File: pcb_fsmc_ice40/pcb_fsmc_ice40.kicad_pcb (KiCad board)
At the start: 2 copper layers, 76.2 x 32 mm, 44 parts, among them P2 CONN_01X20, P3 CONN_01X20, P4 MICRO-SD, P5 CONN_01X12, P6 CONN_01X12, P7 KNUSB, U1 STM32F40X_LQFP144, X1 CRYSTAL

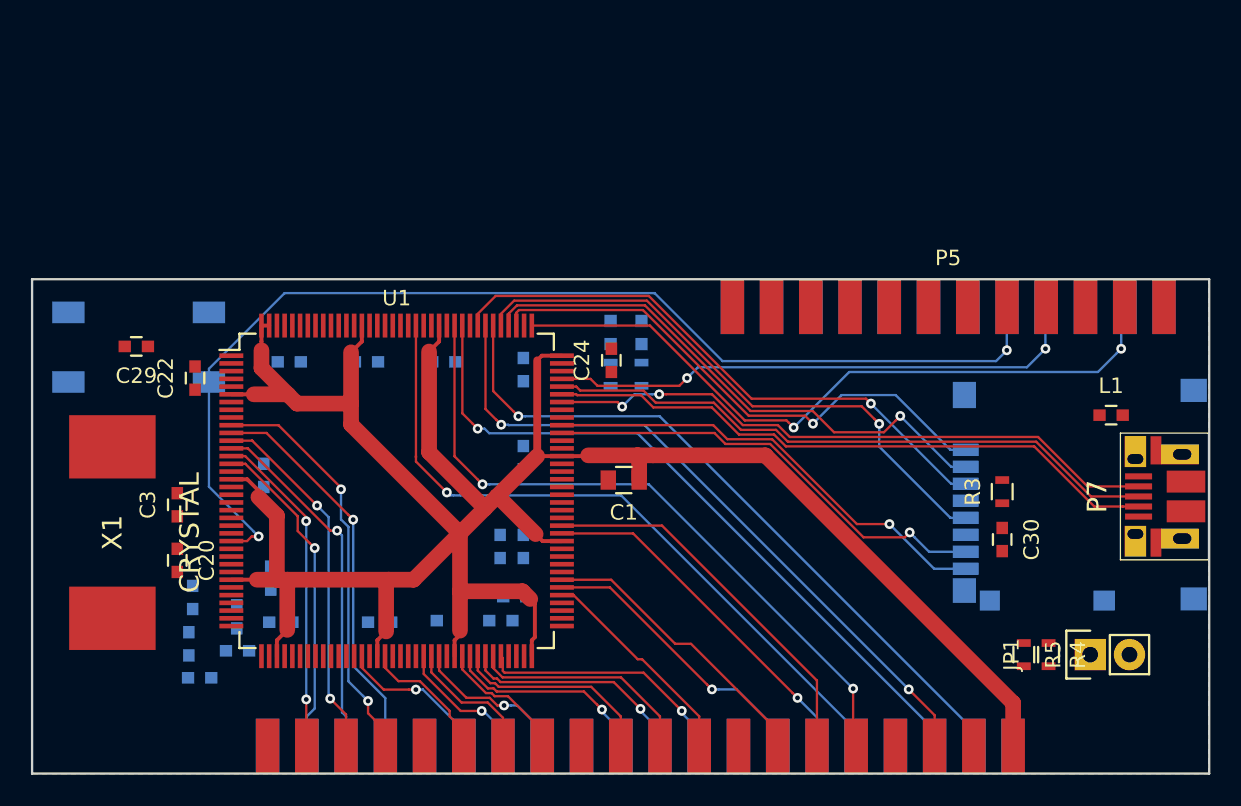
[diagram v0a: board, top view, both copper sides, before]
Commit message: Mostly complete routing.
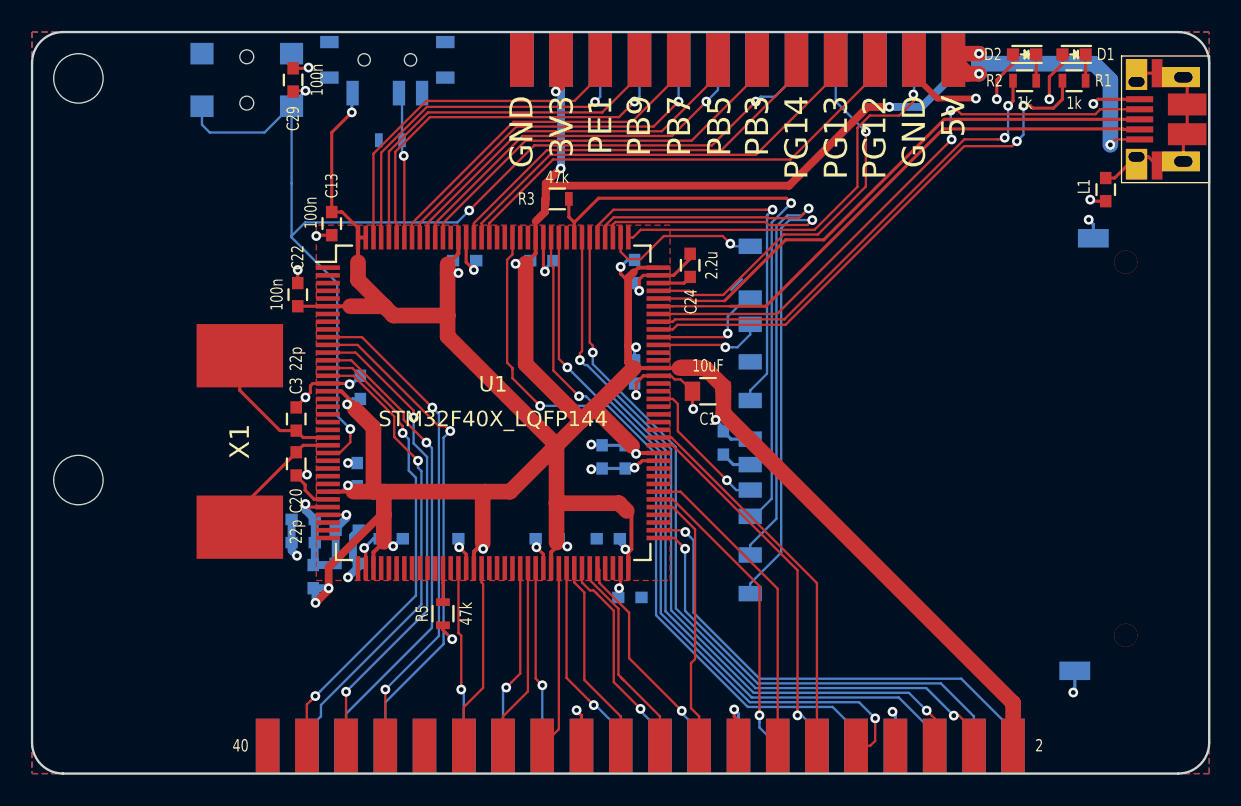
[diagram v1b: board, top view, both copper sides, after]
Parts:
- removed JP1: Jumper_NO_Small, Pin_Headers:Pin_Header_Straight_1x02
- removed P3: CONN_01X20, knielsenlib:ice40_vert_conn
- removed P4: MICRO-SD, knielsenlib:SD_502774
- removed P6: CONN_01X12, knielsenlib:ice40_top_conn_12
- added P1: SD_CARD, knielsenlib:SD_CARD_10100, B.Cu at (170.8, 111.7)
- added REF**: MountingHole_3.2mm_M3, Mounting_Holes:MountingHole_3.2mm_M3, F.Cu at (103.0, 87.0)
- added REF**: MountingHole_3.2mm_M3, Mounting_Holes:MountingHole_3.2mm_M3, F.Cu at (103.0, 113.0)
- added SW1: SWITCH_INV, knielsenlib:switch_msk_12c02, B.Cu at (123.0, 85.8)
- B1: footprint knielsenlib:SWITCH_FSMJSMA -> knielsenlib:pushbutton_EVQ_PSR02K
- C13, D1, D2, R1, R2: moved to F.Cu
- C30, R4: moved to B.Cu
- P2: value CONN_01X20 -> CONN_02X20; moved to F.Cu
- P5: value CONN_01X12 -> CONN_02X12
- moved R4 54.1 mm to (123.2, 91.0), turned to 180 degrees
- moved R5 37.7 mm to (126.6, 121.7), turned to 90 degrees
- moved R3 34.5 mm to (134.0, 94.8), turned to 0 degrees
- moved R1 33.8 mm to (167.4, 87.2), turned to 0 degrees
- moved D1 33.3 mm to (167.4, 85.5), turned to 180 degrees
- moved R2 32.9 mm to (164.2, 87.2), turned to 0 degrees
- moved D2 32.3 mm to (164.2, 85.5), turned to 180 degrees
- moved P7 24.4 mm to (174.5, 89.7)
- moved P5 21.0 mm to (145.7, 85.8), turned to 0 degrees
- moved C29 20.0 mm to (116.9, 87.1), turned to 90 degrees
- moved C30 19.1 mm to (144.8, 110.6)
- moved B1 18.7 mm to (113.9, 87.1), turned to 90 degrees
- moved L1 14.6 mm to (169.5, 94.2), turned to 90 degrees
- moved X1 10.1 mm to (113.5, 110.5)
- moved C20 9.92 mm to (117.1, 112.0)
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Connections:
- P2 pad 10: /sram_d10 -> /sram_we
- P2 pad 11: /sram_d8 -> /sram_d0
- P2 pad 12: GND -> /sram_d1
- P2 pad 13: /sram_d6 -> /sram_d14
- P2 pad 14: /sram_d4 -> /sram_d15
- P2 pad 15: /sram_a6 -> GND
- P2 pad 17: /sram_a1 -> /sram_d12
- P2 pad 18: /sram_a3 -> /sram_d13
- P2 pad 19: /sram_a5 -> /sram_d10
- P2 pad 2: /sram_d2 -> +3.3V
- P2 pad 20: GND -> /sram_d11
- P2 pad 3: /sram_oe -> /fpga_io1
- P2 pad 4: GND -> /sram_d2
- P2 pad 5: /sram2_ce -> /sram_oe
- P2 pad 6: /sram_d0 -> /sram_d3
- P2 pad 7: /sram_d14 -> GND
- P2 pad 9: /sram_d12 -> /sram2_ce
- P5 pad 1: Net-(P5-Pad1) -> GND
- P5 pad 10: Net-(P5-Pad10) -> /pb7
- P5 pad 11: Net-(P5-Pad11) -> /pb4
- P5 pad 12: Net-(P5-Pad12) -> /pb5
- P5 pad 2: Net-(P5-Pad2) -> GND
- P5 pad 3: Net-(P5-Pad3) -> +3.3V
- P5 pad 4: Net-(P5-Pad4) -> +3.3V
- P5 pad 5: Net-(P5-Pad5) -> /pe0
- P5 pad 6: Net-(P5-Pad6) -> /pe1
- P5 pad 7: Net-(P5-Pad7) -> /pb8
- P5 pad 8: Net-(P5-Pad8) -> /pb9
- P5 pad 9: Net-(P5-Pad9) -> /pb6
- R1 pad 1: +3.3V -> /user_led1
- R2 pad 1: /user_led -> /user_led2
- R4 pad 1: GND -> /boot0
- R4 pad 2: /boot0 -> GND
- U1 pad 100: /pa8 -> /user_led1
- U1 pad 101: /pa9 -> /user_led2
- U1 pad 110: /pa15 -> /sd_wp
- U1 pad 127: /sram4_ce -> /pg12
- U1 pad 132: /user_led -> /pg15
- U1 pad 133: /swo -> /pb3
- U1 pad 141: /sram_ble -> /pe0
- U1 pad 142: /sram_bhe -> /pe1
- U1 pad 7: /sd_cd -> /pc13
- U1 pad 73: /pb12 -> /fpga_io1
- U1 pad 74: /pb13 -> /fpga_io2
- U1 pad 8: /sd_wp -> /pc14
- U1 pad 91: /pg6 -> /sd_cd
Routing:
- net +3.3V: track 157.9 -> 250.6 mm, vias 0 -> 19
- net GND: track 0.00 -> 80.6 mm, vias 0 -> 30
- net /user_led1: track 0.00 -> 34.7 mm, vias 0 -> 2
- net /fpga_io2: track 0.00 -> 32.1 mm, vias 0 -> 1
- net /user_led2: track 0.00 -> 31.3 mm, vias 0 -> 2
- net /pg12: track 0.00 -> 30.8 mm
- net /fpga_io1: track 0.00 -> 29.5 mm, vias 0 -> 1
- net /pg13: track 0.00 -> 28.8 mm
- net /pg14: track 0.00 -> 26.8 mm
- net /pb3: track 0.00 -> 26.2 mm
- net /pb8: track 0.00 -> 25.2 mm, vias 0 -> 1
- net /pb9: track 0.00 -> 24.8 mm
- net /pb4: track 0.00 -> 24.7 mm, vias 0 -> 1
- net /pb5: track 0.00 -> 24.7 mm
- net /pb6: track 0.00 -> 23.6 mm, vias 0 -> 1
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- added copper zone on F.Cu, net +3.3V
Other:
- board size 76.2 x 32 mm -> 76.2 x 48 mm
- board text added: "1"
- board text added: "2"
- board text added: "39"
- board text added: "3V3"
- board text added: "40"
- board text added: "5V"
- board text added: "GND"
- board text added: "NRST"
- board text added: "PB3"
- board text added: "PB4"
- board text added: "PB5"
- board text added: "PB6"
- board text added: "PB7"
- board text added: "PB8"
- board text added: "PB9"
- board text added: "PE0"
- board text added: "PE1"
- board text added: "PG12"
- board text added: "PG13"
- board text added: "PG14"
- board text added: "SWCLK"
- board text added: "SWD"
- board text added: "SWDIO"
